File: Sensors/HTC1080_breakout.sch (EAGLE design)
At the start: 4 parts

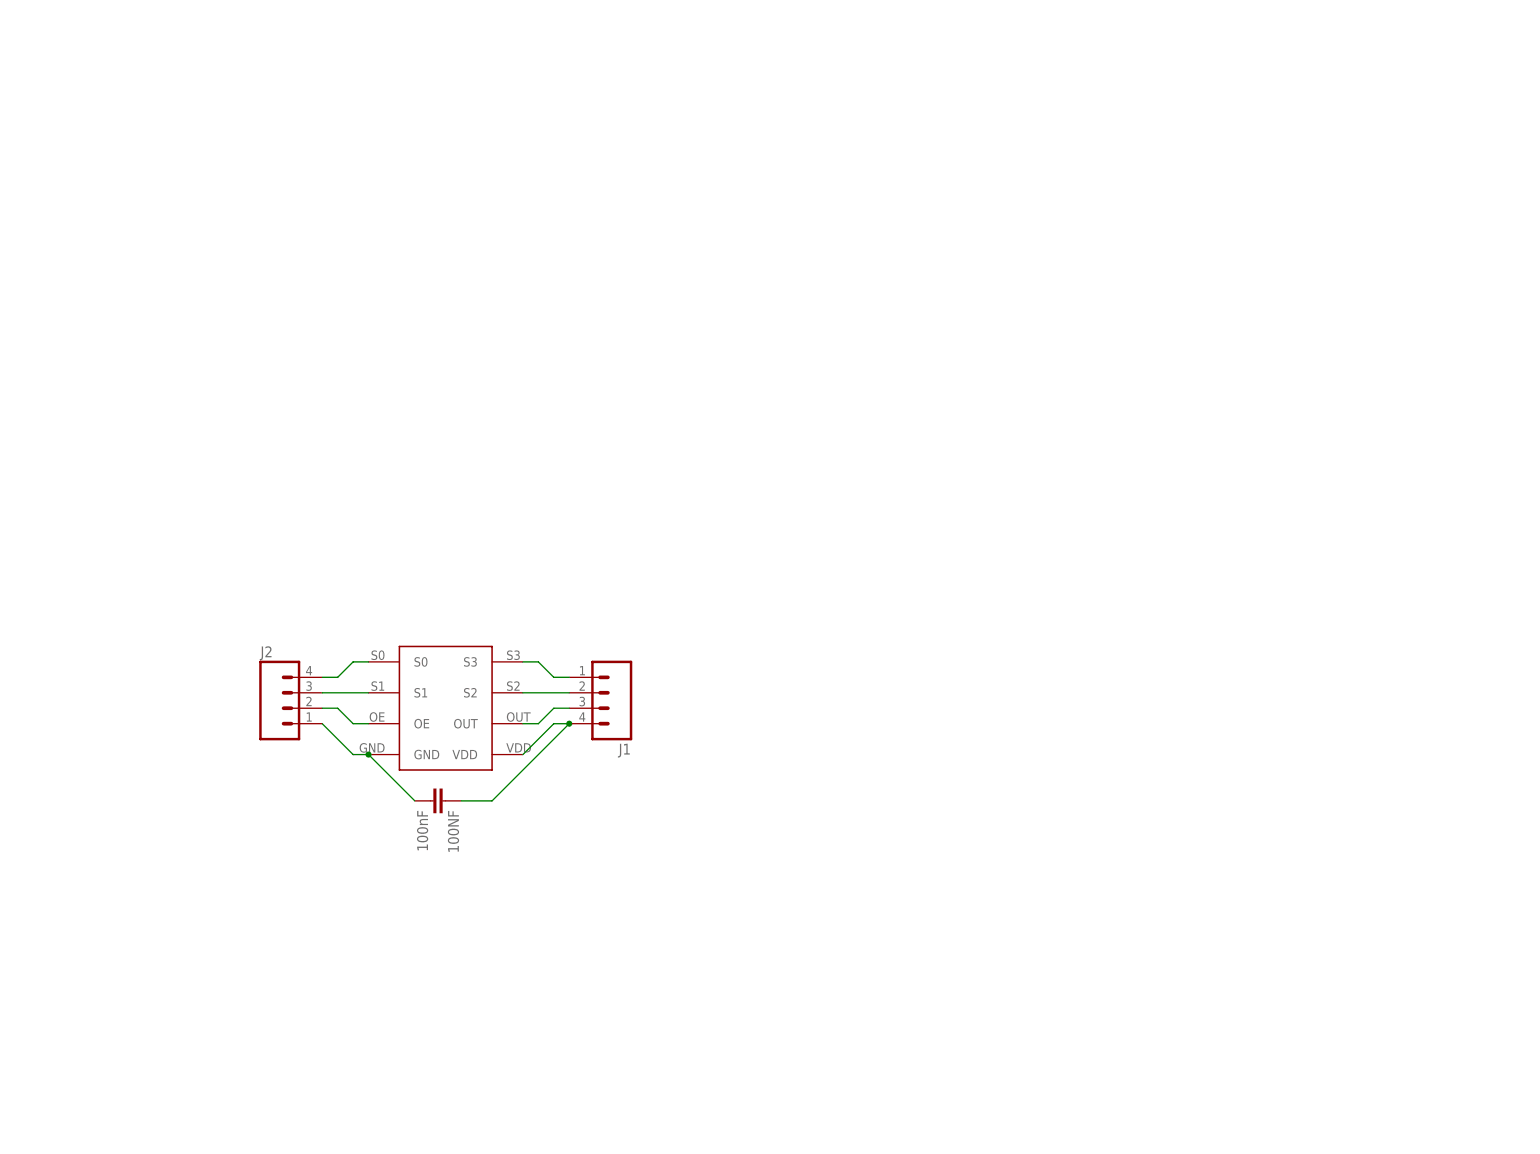
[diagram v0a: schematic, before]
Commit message: new boards
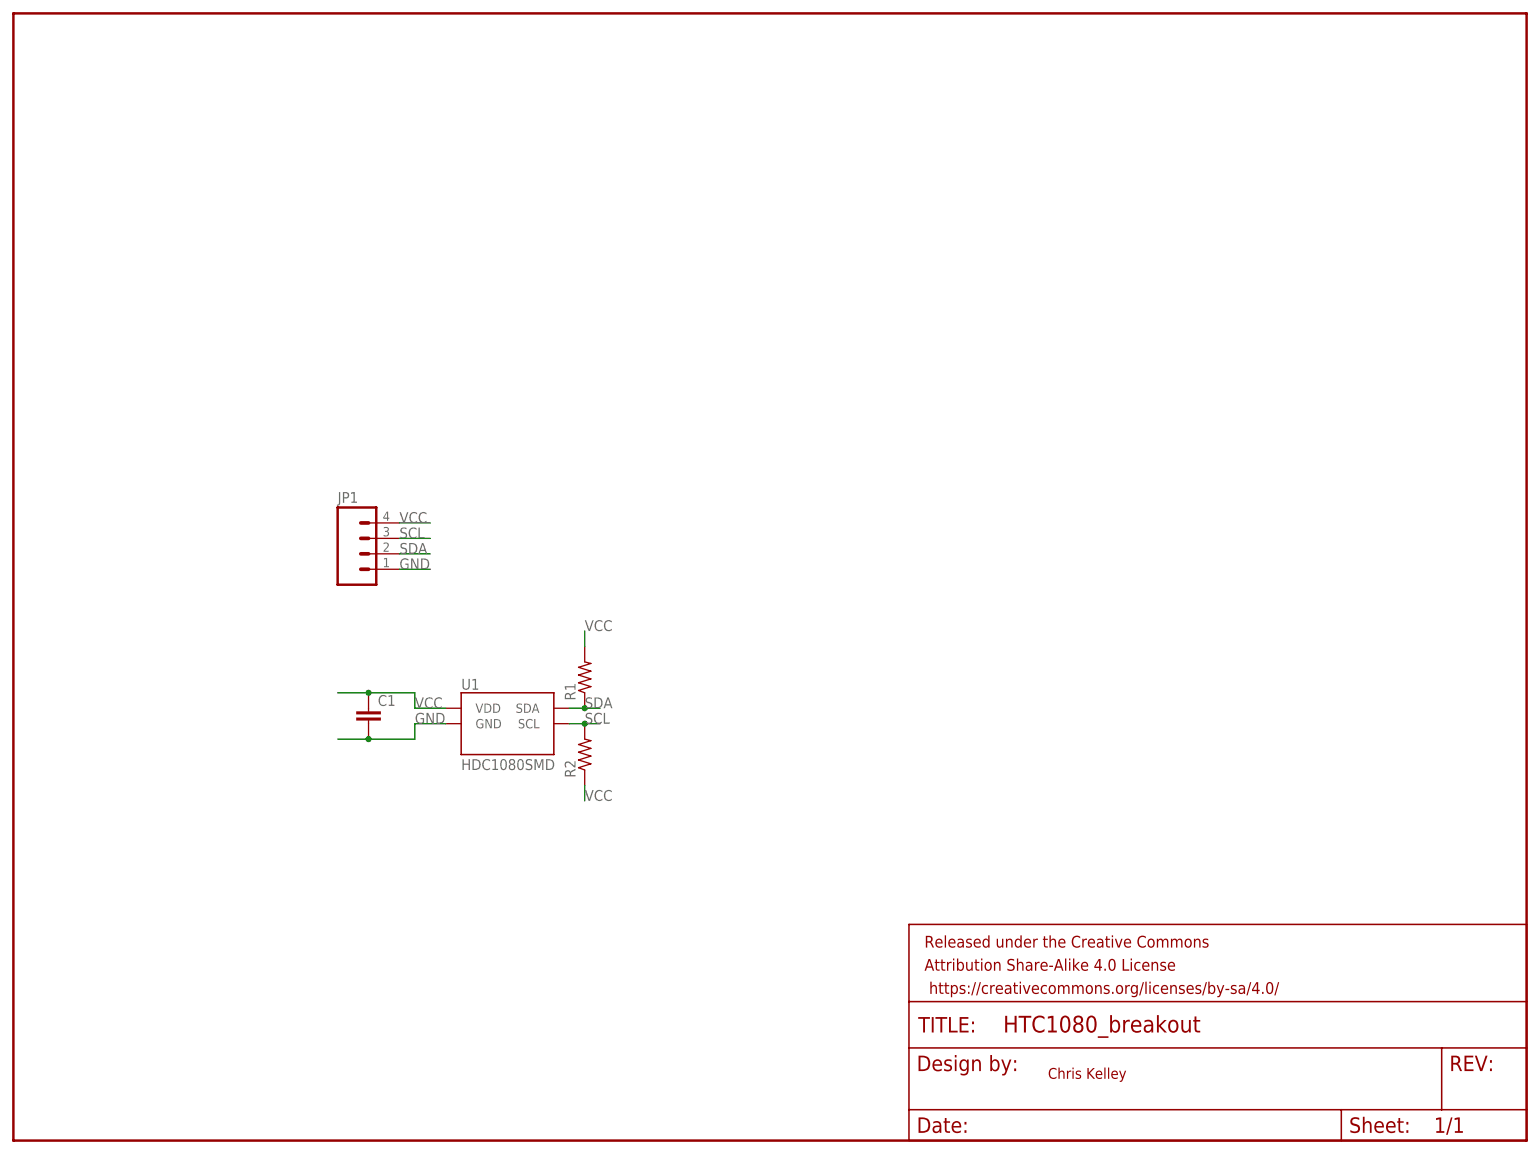
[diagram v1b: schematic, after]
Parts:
- removed 100NF: 100nF, SparkFun-Capacitors:CAP0603-CAP
- removed J1, J2: (no value), SparkFun-Connectors:M04PTH
- removed U$1: TSL230RDSMD, awqua_eagle_library:TSL230RDSMD
- added C1: (no value), SparkFun-Passives:CAP0603-CAP
- added FRAME1: FRAME-LETTER, SparkFun-Aesthetics:FRAME-LETTER
- added JP1: (no value), SparkFun-Connectors:M04PTH
- added R1, R2: (no value), SparkFun-Passives:RESISTOR0603-RES
- added U1: HDC1080SMD, adam-sensors:HDC1080SMD
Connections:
- removed net N$1: J2.4, U$1.S0
- removed net N$2: J2.3, U$1.S1
- removed net N$3: J2.2, U$1.OE
- removed net N$5: J1.1, U$1.S3
- removed net N$6: J1.2, U$1.S2
- removed net N$7: J1.3, U$1.OUT
- removed net N$8: 100NF.1, J1.4, U$1.VDD
- new net SCL: JP1.3, R2.2, U1.SCL
- new net SDA: JP1.2, R1.1, U1.SDA
- new net VCC: C1.1, JP1.4, R1.2, R2.1, U1.VDD
- net GND: now also C1.2, JP1.1, U1.GND; no longer 100NF.2, J2.1, U$1.GND
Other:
- note added: "Chris Kelley"
